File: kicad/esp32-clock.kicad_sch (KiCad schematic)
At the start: 19 parts, among them J1 Conn_01x07_Socket, SW1 RESET, SW2 BOOT, U1 ESP32-PICO-V3

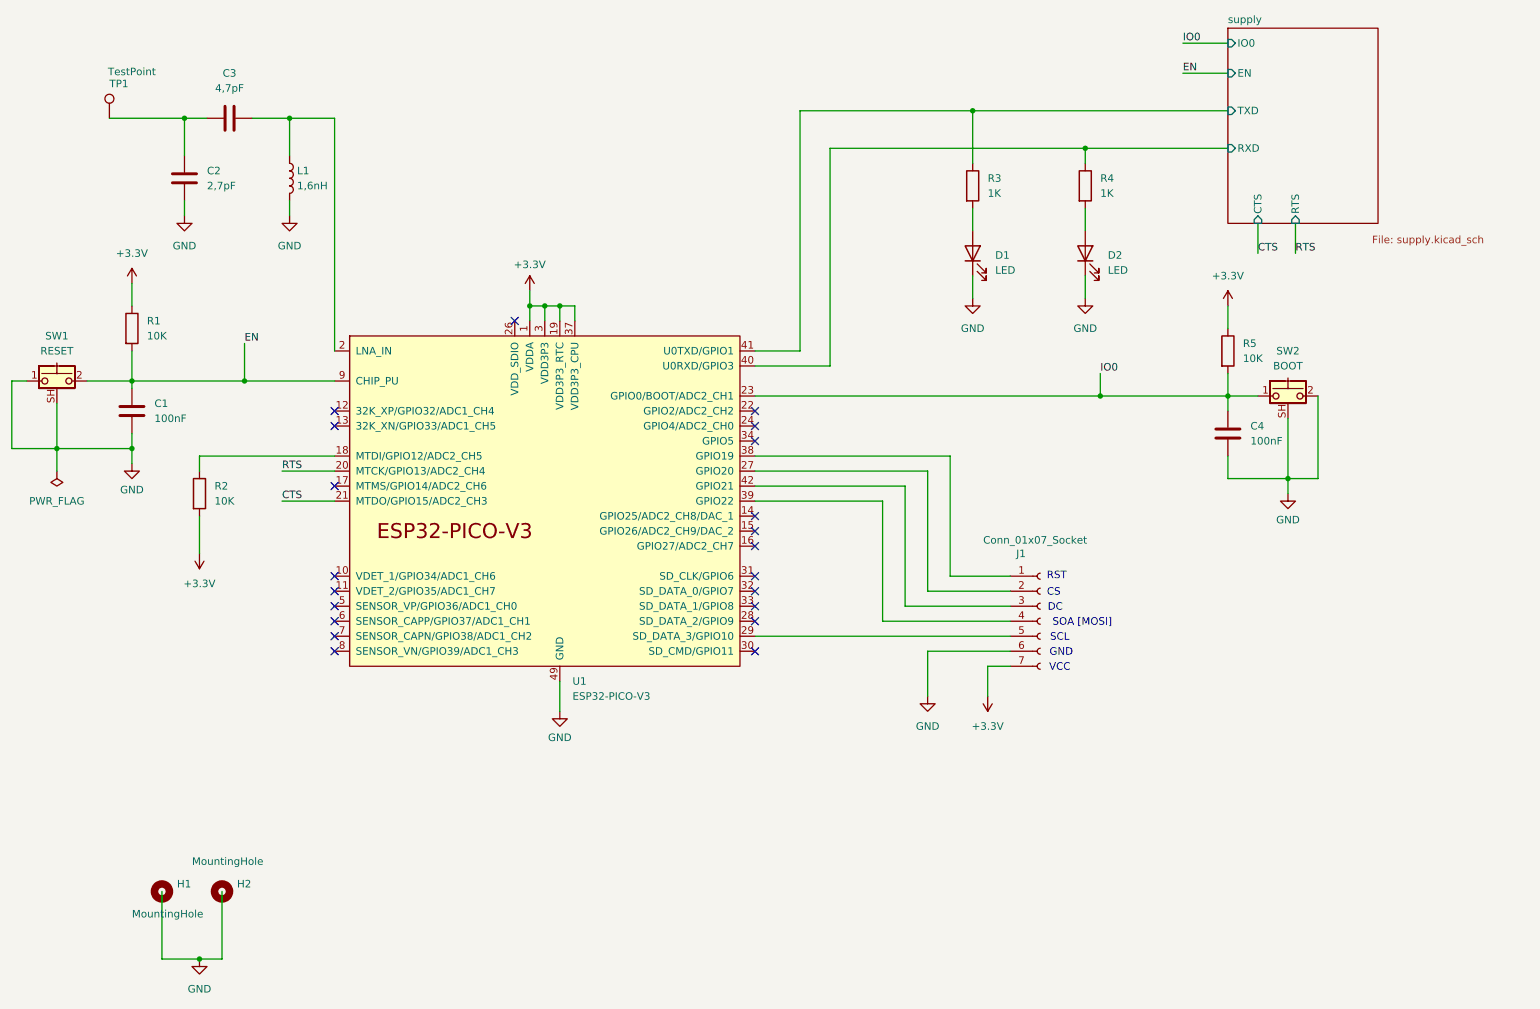
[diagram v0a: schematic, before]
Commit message: init
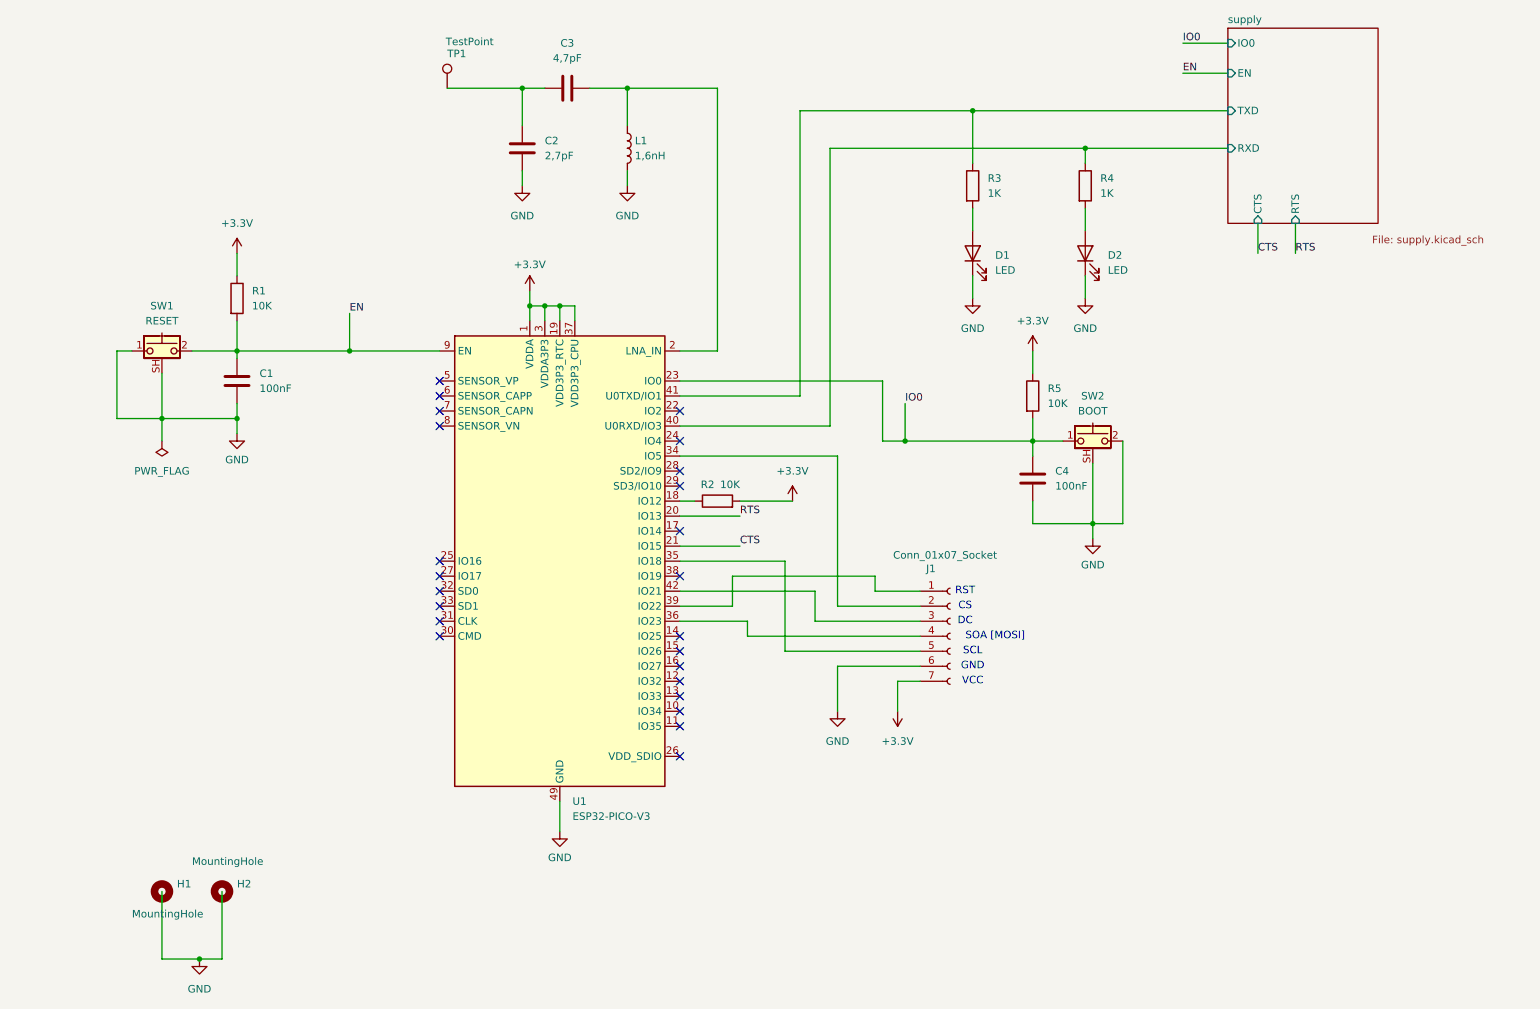
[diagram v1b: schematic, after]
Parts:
- removed U1: ESP32-PICO-V3, Package_DFN_QFN:QFN-48-1EP_7x7mm_P0.5mm_EP5.15x5.15mm, symbol PCM_Espressif:ESP32-PICO-V3
- added U1: ESP32-PICO-V3, Package_DFN_QFN:QFN-48-1EP_7x7mm_P0.5mm_EP5.3x5.3mm, symbol MCU_Espressif:ESP32-PICO-V3
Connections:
- net +3.3V: now also U1.1 (VDDA), U1.19 (VDD3P3_RTC), U1.3 (VDDA3P3), U1.37 (VDD3P3_CPU), U1.4 (VDDA3P3), U1.43 (VDDA), U1.46 (VDDA)
- net CTS: now also U1.21 (IO15)
- net EN: now also U1.9 (EN)
- net GND: now also U1.49 (GND)
- net IO0: now also U1.23 (IO0)
- net RTS: now also U1.20 (IO13)
- net supply/RXD: now also U1.40 (U0RXD/IO3)
- net supply/TXD: now also U1.41 (U0TXD/IO1)
- net at C3.2, L1.1: now also U1.2 (LNA_IN)
- net at R2.1: now also U1.18 (IO12)
- net at J1.2 (Pin_2): now also U1.34 (IO5)
- net at J1.5 (Pin_5): now also U1.35 (IO18)
- net at J1.1 (Pin_1): now also U1.39 (IO22)
- net at J1.4 (Pin_4): now also U1.36 (IO23)
- net at J1.3 (Pin_3): now also U1.42 (IO21)
- no-connect marks 21 -> 24
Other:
- moved on the sheet: C1, C2, C3, C4, J1, L1, R1, R2, R5, SW1, SW2, TP1
